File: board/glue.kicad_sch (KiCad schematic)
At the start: 9 parts, among them J1 Conn_01x05_Pin, Q2 PN2222A, U12 GLUE

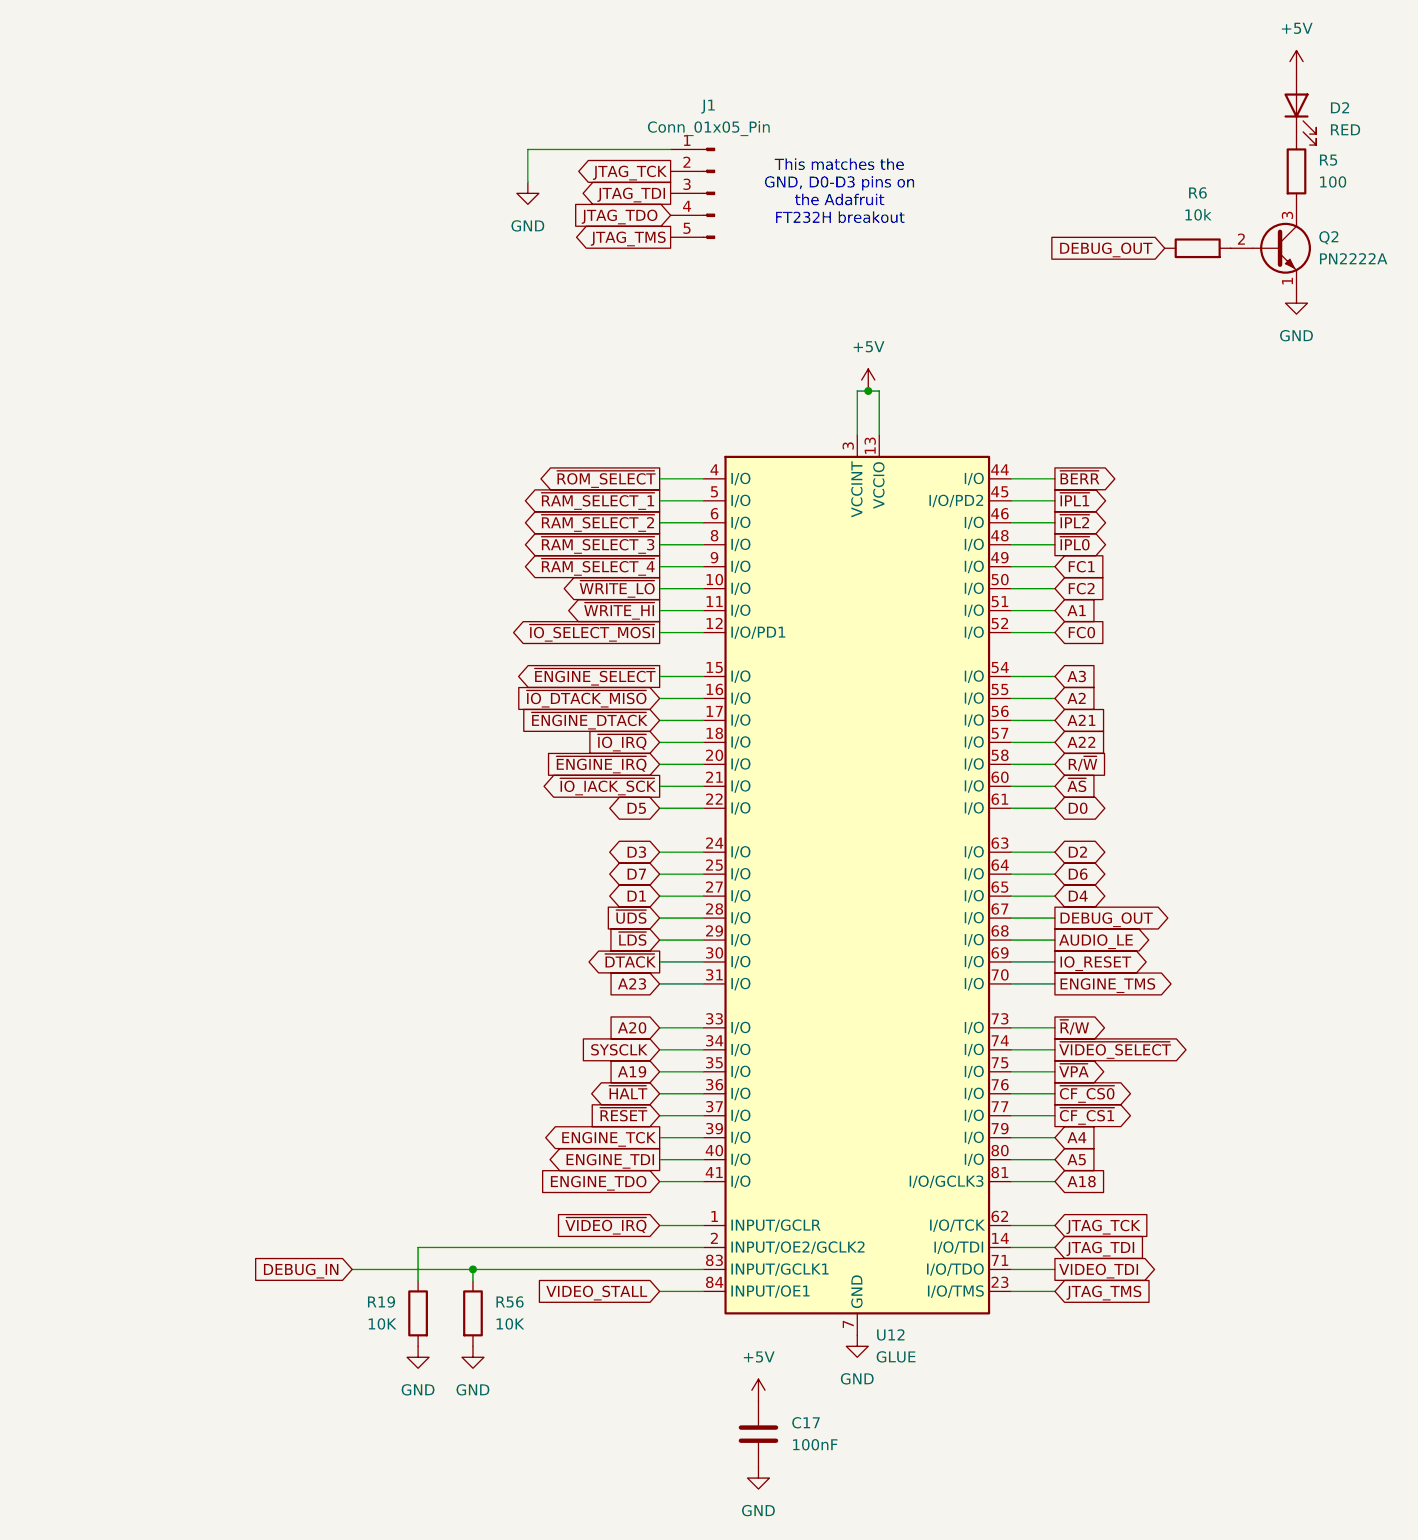
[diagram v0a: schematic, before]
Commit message: checkpoint
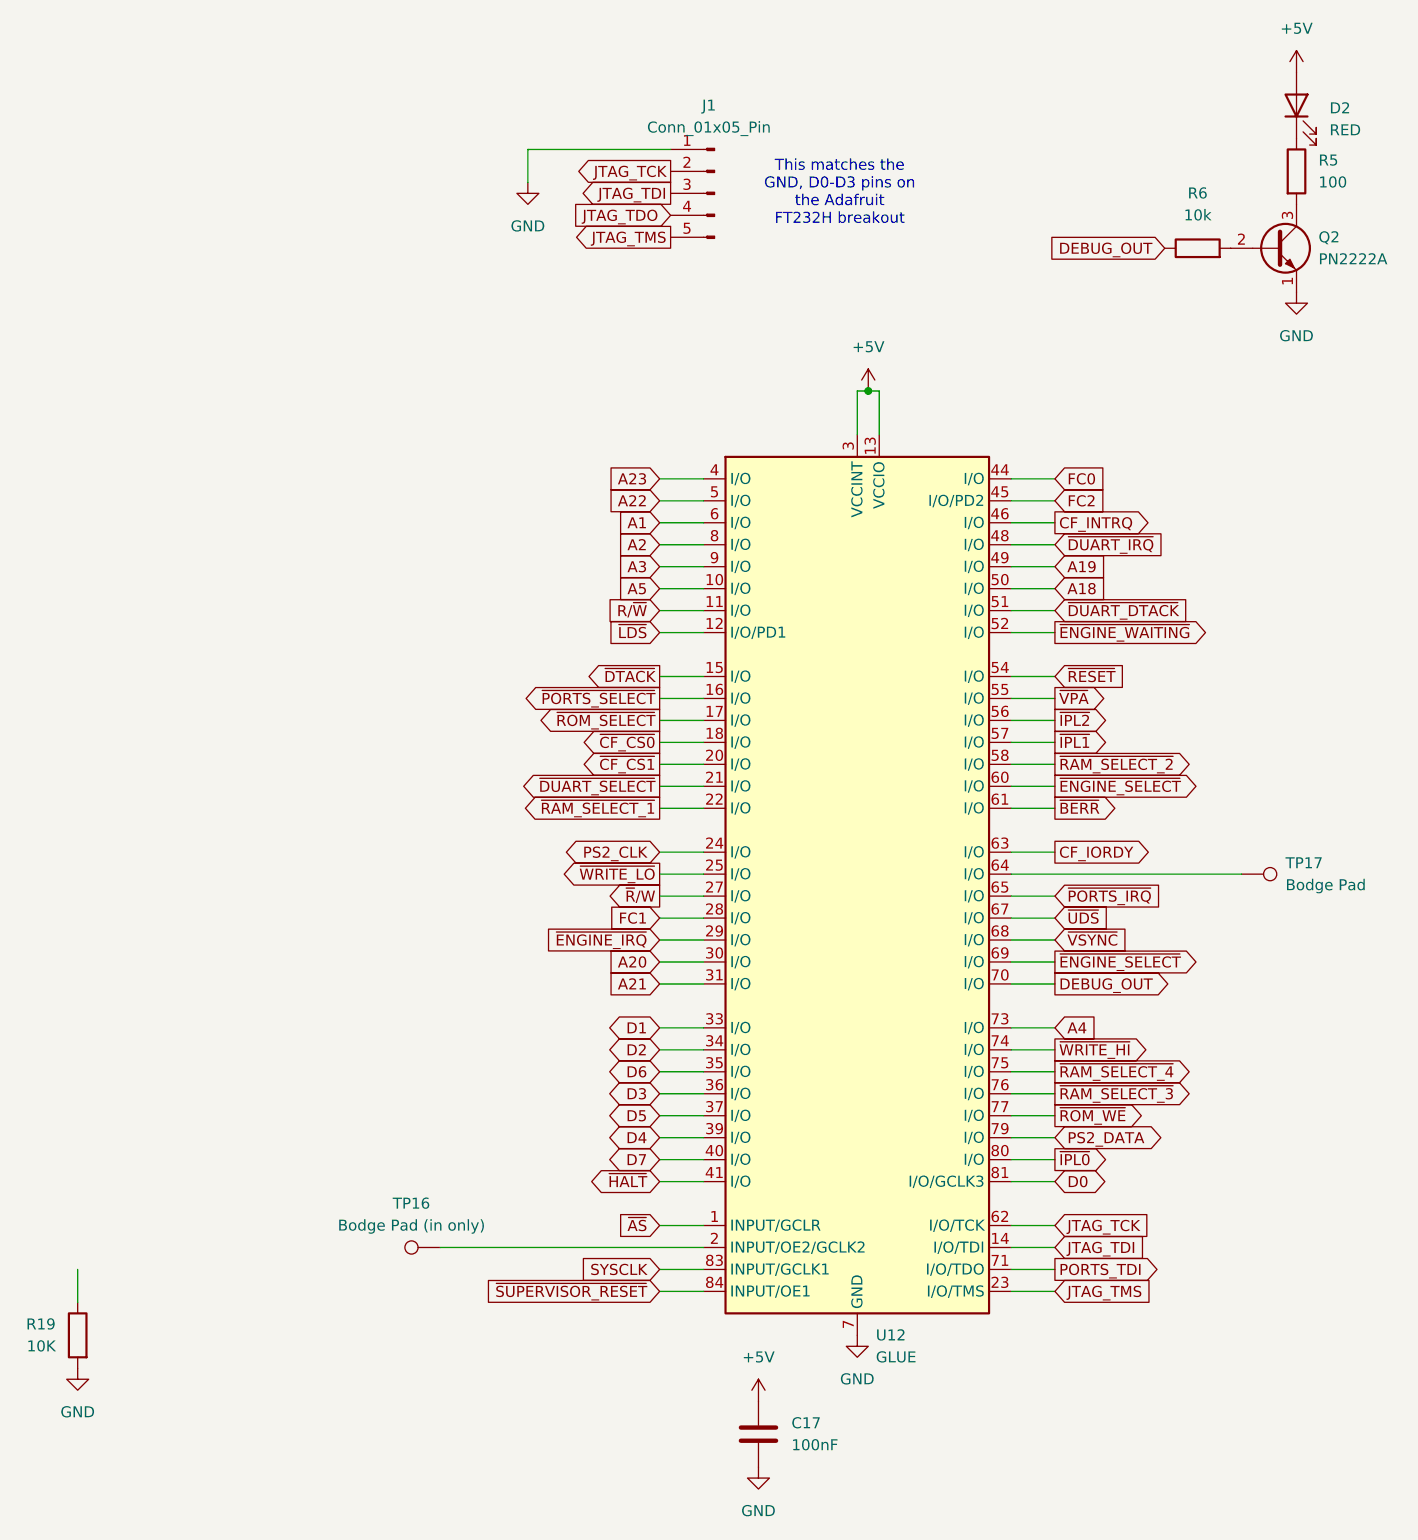
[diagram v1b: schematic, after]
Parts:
- removed R56: 10K, Resistor_THT:R_Axial_DIN0207_L6.3mm_D2.5mm_P10.16mm_Horizontal, symbol Device:R
- added TP16: Bodge Pad (in only), symbol Connector:TestPoint
- added TP17: Bodge Pad, symbol Connector:TestPoint
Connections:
- net DEBUG_IN is gone; now on net SYSCLK: U12.83 (INPUT/GCLK1)
- net ENGINE_TCK is gone; now on net D4: U12.39 (I/O)
- net ENGINE_TDI is gone; now on net D7: U12.40 (I/O)
- net ENGINE_TDO is gone; now on net ~{HALT}: U12.41 (I/O)
- net ENGINE_TMS is gone; now on net DEBUG_OUT: U12.70 (I/O)
- net IO_RESET is gone; now on net ~{ENGINE_SELECT}: U12.69 (I/O)
- net ~{ENGINE_DTACK} is gone; now on net ~{ROM_SELECT}: U12.17 (I/O)
- net ~{IO_IRQ} is gone; now on net ~{CF_CS0}: U12.18 (I/O)
- net ~{IO_SELECT_MOSI} is gone; now on net ~{LDS}: U12.12 (I/O/PD1)
- net ~{VIDEO_IRQ} is gone; now on net ~{AS}: U12.1 (INPUT/GCLR)
- net ~{VIDEO_SELECT} is gone; now on net ~{WRITE_HI}: U12.74 (I/O)
- net A1: now also U12.6 (I/O); no longer U12.51 (I/O)
- net A18: now also U12.50 (I/O); no longer U12.81 (I/O/GCLK3)
- net A19: now also U12.49 (I/O); no longer U12.35 (I/O)
- net A2: now also U12.8 (I/O); no longer U12.55 (I/O)
- net A20: now also U12.30 (I/O); no longer U12.33 (I/O)
- net A21: now also U12.31 (I/O); no longer U12.56 (I/O)
- net A22: now also U12.5 (I/O); no longer U12.57 (I/O)
- net A23: now also U12.4 (I/O); no longer U12.31 (I/O)
- net A3: now also U12.9 (I/O); no longer U12.54 (I/O)
- net A4: now also U12.73 (I/O); no longer U12.79 (I/O)
- net A5: now also U12.10 (I/O); no longer U12.80 (I/O)
- net D0: now also U12.81 (I/O/GCLK3); no longer U12.61 (I/O)
- net D1: now also U12.33 (I/O); no longer U12.27 (I/O)
- net D2: now also U12.34 (I/O); no longer U12.63 (I/O)
- net D3: now also U12.36 (I/O); no longer U12.24 (I/O)
- net D4: no longer U12.65 (I/O)
- net D5: now also U12.37 (I/O); no longer U12.22 (I/O)
- net D6: now also U12.35 (I/O); no longer U12.64 (I/O)
- net D7: no longer U12.25 (I/O)
- net DEBUG_OUT: no longer U12.67 (I/O)
- net FC0: now also U12.44 (I/O); no longer U12.52 (I/O)
- net FC1: now also U12.28 (I/O); no longer U12.49 (I/O)
- net FC2: now also U12.45 (I/O/PD2); no longer U12.50 (I/O)
- net R/~{W}: now also U12.11 (I/O); no longer U12.58 (I/O)
- net SYSCLK: no longer U12.34 (I/O)
- net ~{AS}: no longer U12.60 (I/O)
- net ~{BERR}: now also U12.61 (I/O); no longer U12.44 (I/O)
- net ~{CF_CS0}: no longer U12.76 (I/O)
- net ~{CF_CS1}: now also U12.20 (I/O); no longer U12.77 (I/O)
- net ~{DTACK}: now also U12.15 (I/O); no longer U12.30 (I/O)
- net ~{ENGINE_IRQ}: now also U12.29 (I/O); no longer U12.20 (I/O)
- net ~{ENGINE_SELECT}: now also U12.60 (I/O); no longer U12.15 (I/O)
- net ~{HALT}: no longer U12.36 (I/O)
- net ~{IPL0}: now also U12.80 (I/O); no longer U12.48 (I/O)
- net ~{IPL1}: now also U12.57 (I/O); no longer U12.45 (I/O/PD2)
- net ~{IPL2}: now also U12.56 (I/O); no longer U12.46 (I/O)
- net ~{LDS}: no longer U12.29 (I/O)
- net ~{RAM_SELECT_1}: now also U12.22 (I/O); no longer U12.5 (I/O)
- net ~{RAM_SELECT_2}: now also U12.58 (I/O); no longer U12.6 (I/O)
- net ~{RAM_SELECT_3}: now also U12.76 (I/O); no longer U12.8 (I/O)
- net ~{RAM_SELECT_4}: now also U12.75 (I/O); no longer U12.9 (I/O)
- net ~{RESET}: now also U12.54 (I/O); no longer U12.37 (I/O)
- net ~{ROM_SELECT}: no longer U12.4 (I/O)
- net ~{R}/W: now also U12.27 (I/O); no longer U12.73 (I/O)
- net ~{UDS}: now also U12.67 (I/O); no longer U12.28 (I/O)
- net ~{VPA}: now also U12.55 (I/O); no longer U12.75 (I/O)
- net ~{WRITE_HI}: no longer U12.11 (I/O)
- net ~{WRITE_LO}: now also U12.25 (I/O); no longer U12.10 (I/O)
- net at U12.2 (INPUT/OE2/GCLK2): now also TP16.1; no longer R19.1
- net AUDIO_LE renamed ~{VSYNC}
- net VIDEO_STALL renamed ~{SUPERVISOR_RESET}
- net VIDEO_TDI renamed PORTS_TDI
- net ~{IO_DTACK_MISO} renamed ~{PORTS_SELECT}
- net ~{IO_IACK_SCK} renamed ~{DUART_SELECT}
- new net: TP17.1, U12.64 (I/O)
- new net CF_INTRQ: U12.46 (I/O)
- new net CF_IORDY: U12.63 (I/O)
- new net PS2_CLK: U12.24 (I/O)
- new net PS2_DATA: U12.79 (I/O)
- new net ~{DUART_DTACK}: U12.51 (I/O)
- new net ~{DUART_IRQ}: U12.48 (I/O)
- new net ~{ENGINE_WAITING}: U12.52 (I/O)
- new net ~{PORTS_IRQ}: U12.65 (I/O)
- new net ~{ROM_WE}: U12.77 (I/O)
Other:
- moved on the sheet: R19

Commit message: checkpoint
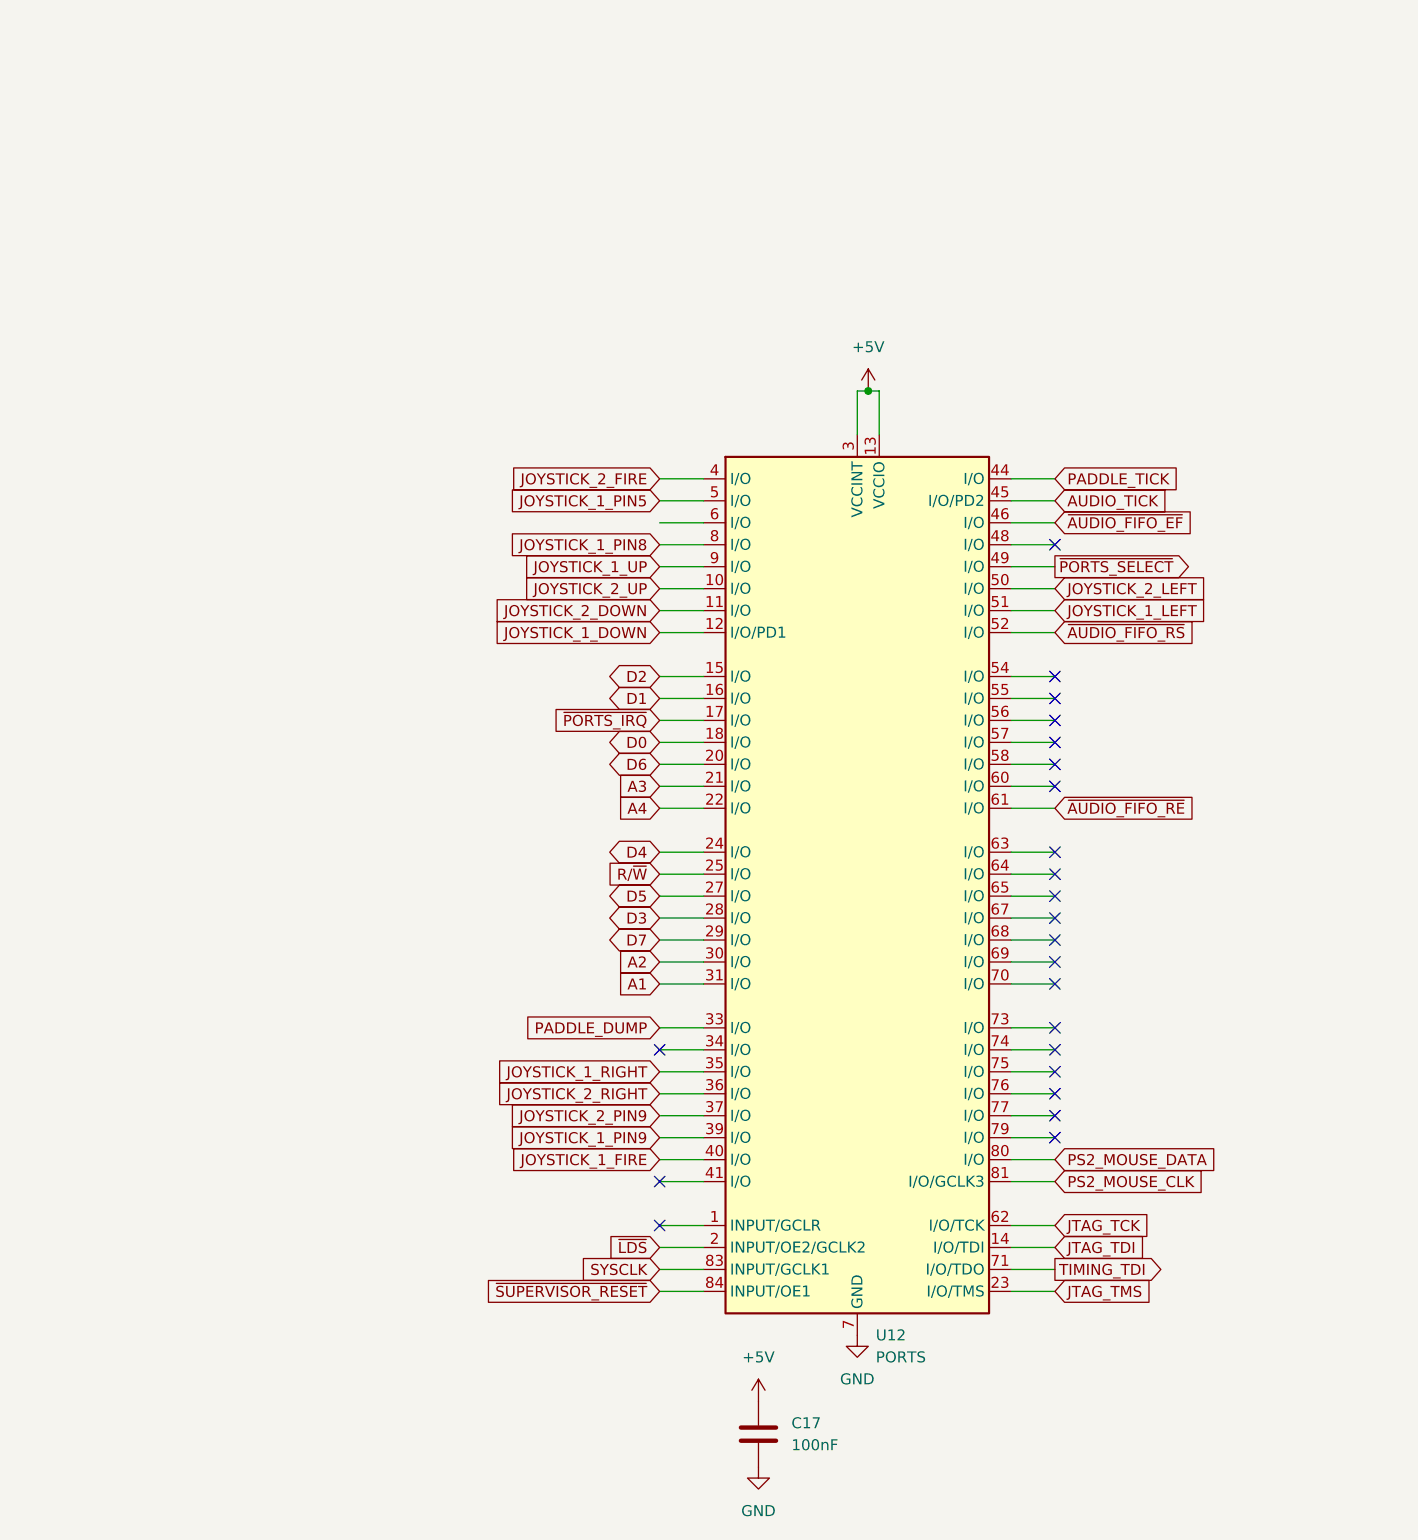
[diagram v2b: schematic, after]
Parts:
- removed D2: RED, LED_THT:LED_D3.0mm, symbol Device:LED
- removed J1: Conn_01x05_Pin, Connector_PinHeader_2.54mm:PinHeader_1x05_P2.54mm_Vertical, symbol Connector:Conn_01x05_Pin
- removed Q2: PN2222A, Package_TO_SOT_THT:TO-92_Inline, symbol Transistor_BJT:PN2222A
- removed R19: 10K, Resistor_THT:R_Axial_DIN0207_L6.3mm_D2.5mm_P10.16mm_Horizontal, symbol Device:R
- removed R5: 100, Resistor_THT:R_Axial_DIN0207_L6.3mm_D2.5mm_P10.16mm_Horizontal, symbol Device:R
- removed R6: 10k, Resistor_THT:R_Axial_DIN0207_L6.3mm_D2.5mm_P10.16mm_Horizontal, symbol Device:R
- removed TP16: Bodge Pad (in only), symbol Connector:TestPoint
- removed TP17: Bodge Pad, symbol Connector:TestPoint
- U12: value GLUE -> PORTS
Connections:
- net A19 is gone; now on net ~{PORTS_SELECT}: U12.49 (I/O)
- net A20 is gone; now on net A2: U12.30 (I/O)
- net A21 is gone; now on net A1: U12.31 (I/O)
- net FC1 is gone; now on net D3: U12.28 (I/O)
- net PS2_CLK is gone; now on net D4: U12.24 (I/O)
- net ~{CF_CS0} is gone; now on net D0: U12.18 (I/O)
- net ~{CF_CS1} is gone; now on net D6: U12.20 (I/O)
- net ~{DTACK} is gone; now on net D2: U12.15 (I/O)
- net ~{DUART_SELECT} is gone; now on net A3: U12.21 (I/O)
- net ~{ENGINE_IRQ} is gone; now on net D7: U12.29 (I/O)
- net ~{RAM_SELECT_1} is gone; now on net A4: U12.22 (I/O)
- net ~{ROM_SELECT} is gone; now on net ~{PORTS_IRQ}: U12.17 (I/O)
- net ~{R}/W is gone; now on net D5: U12.27 (I/O)
- net ~{WRITE_LO} is gone; now on net R/~{W}: U12.25 (I/O)
- net A1: no longer U12.6 (I/O)
- net A2: no longer U12.8 (I/O)
- net A3: no longer U12.9 (I/O)
- net A4: no longer U12.73 (I/O)
- net D0: no longer U12.81 (I/O/GCLK3)
- net D1: now also U12.16 (I/O); no longer U12.33 (I/O)
- net D2: no longer U12.34 (I/O)
- net D3: no longer U12.36 (I/O)
- net D4: no longer U12.39 (I/O)
- net D5: no longer U12.37 (I/O)
- net D6: no longer U12.35 (I/O)
- net D7: no longer U12.40 (I/O)
- net R/~{W}: no longer U12.11 (I/O)
- net ~{LDS}: now also U12.2 (INPUT/OE2/GCLK2); no longer U12.12 (I/O/PD1)
- net ~{PORTS_IRQ}: no longer U12.65 (I/O)
- net ~{PORTS_SELECT}: no longer U12.16 (I/O)
- net A18 renamed JOYSTICK_2_LEFT
- net A22 renamed JOYSTICK_1_PIN5
- net A23 renamed JOYSTICK_2_FIRE
- net A5 renamed JOYSTICK_2_UP
- net CF_INTRQ renamed ~{AUDIO_FIFO_EF}
- net CF_IORDY: no longer names the net of U12.63 (I/O)
- net DEBUG_OUT: no longer names the net of U12.70 (I/O)
- net FC0 renamed PADDLE_TICK
- net FC2 renamed AUDIO_TICK
- net PORTS_TDI renamed TIMING_TDI
- net PS2_DATA: no longer names the net of U12.79 (I/O)
- net ~{AS}: no longer names the net of U12.1 (INPUT/GCLR)
- net ~{BERR} renamed ~{AUDIO_FIFO_RE}
- net ~{DUART_DTACK} renamed JOYSTICK_1_LEFT
- net ~{DUART_IRQ}: no longer names the net of U12.48 (I/O)
- net ~{ENGINE_SELECT}: no longer names the net of U12.60 (I/O)
- net ~{ENGINE_SELECT}: no longer U12.69 (I/O)
- net ~{ENGINE_WAITING} renamed ~{AUDIO_FIFO_RS}
- net ~{HALT}: no longer names the net of U12.41 (I/O)
- net ~{IPL0} renamed PS2_MOUSE_DATA
- net ~{IPL1}: no longer names the net of U12.57 (I/O)
- net ~{IPL2}: no longer names the net of U12.56 (I/O)
- net ~{RAM_SELECT_2}: no longer names the net of U12.58 (I/O)
- net ~{RAM_SELECT_3}: no longer names the net of U12.76 (I/O)
- net ~{RAM_SELECT_4}: no longer names the net of U12.75 (I/O)
- net ~{RESET}: no longer names the net of U12.54 (I/O)
- net ~{ROM_WE}: no longer names the net of U12.77 (I/O)
- net ~{UDS}: no longer names the net of U12.67 (I/O)
- net ~{VPA}: no longer names the net of U12.55 (I/O)
- net ~{VSYNC}: no longer names the net of U12.68 (I/O)
- net ~{WRITE_HI}: no longer names the net of U12.74 (I/O)
- new net JOYSTICK_1_DOWN: U12.12 (I/O/PD1)
- new net JOYSTICK_1_FIRE: U12.40 (I/O)
- new net JOYSTICK_1_PIN8: U12.8 (I/O)
- new net JOYSTICK_1_PIN9: U12.39 (I/O)
- new net JOYSTICK_1_RIGHT: U12.35 (I/O)
- new net JOYSTICK_1_UP: U12.9 (I/O)
- new net JOYSTICK_2_DOWN: U12.11 (I/O)
- new net JOYSTICK_2_PIN9: U12.37 (I/O)
- new net JOYSTICK_2_RIGHT: U12.36 (I/O)
- new net PADDLE_DUMP: U12.33 (I/O)
- new net PS2_MOUSE_CLK: U12.81 (I/O/GCLK3)
- no-connect marks 0 -> 23
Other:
- note removed: "This matches the GND, D0-D3 pins on the Adafruit FT232H breakout"
